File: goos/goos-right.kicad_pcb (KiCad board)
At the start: 2 copper layers, 140.2 x 108.1 mm, 22 parts

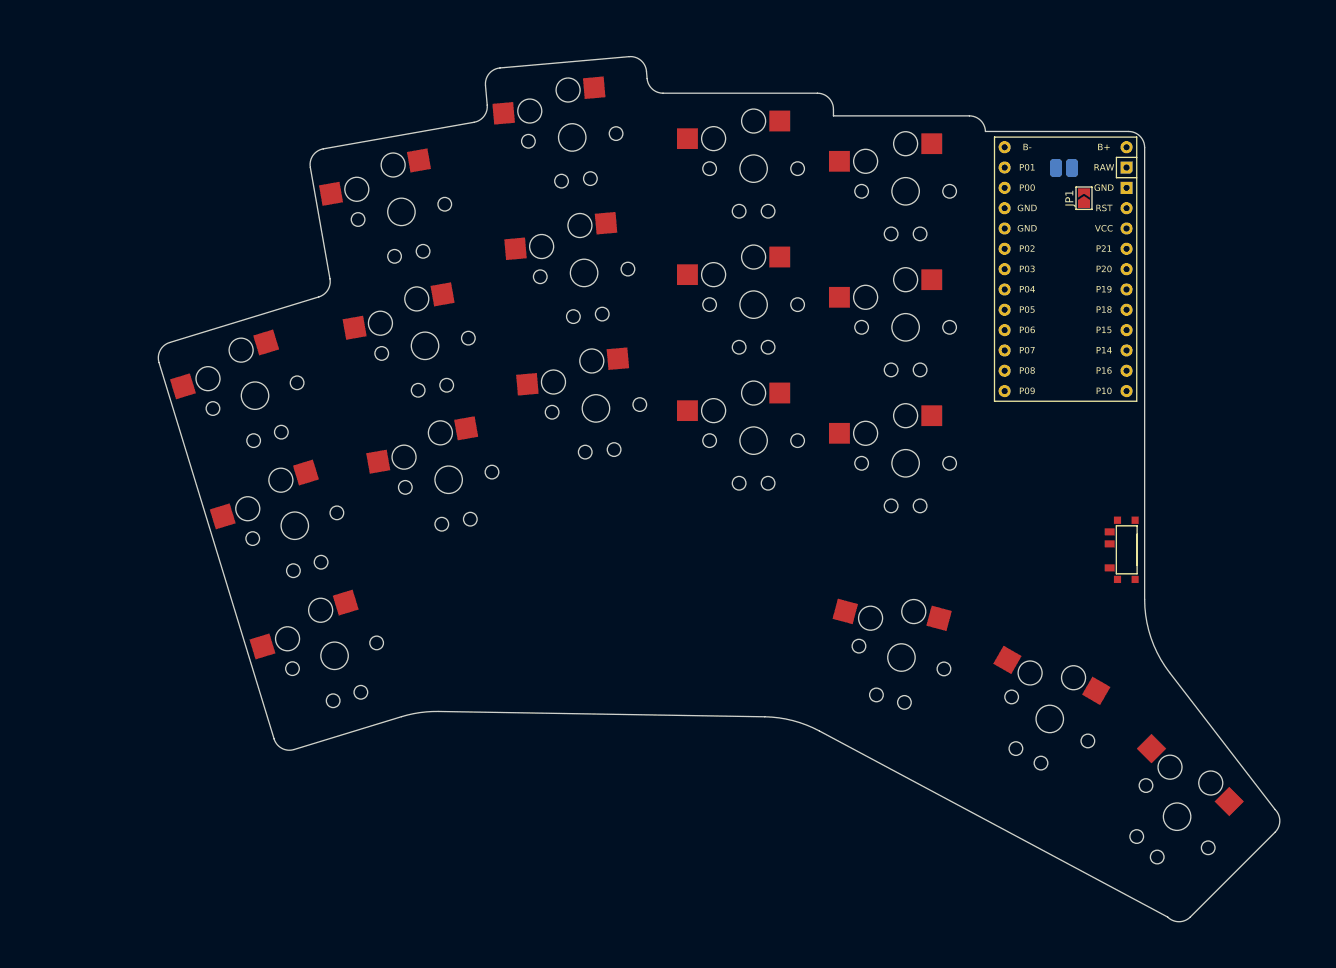
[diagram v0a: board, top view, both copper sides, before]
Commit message: feat: right side routed
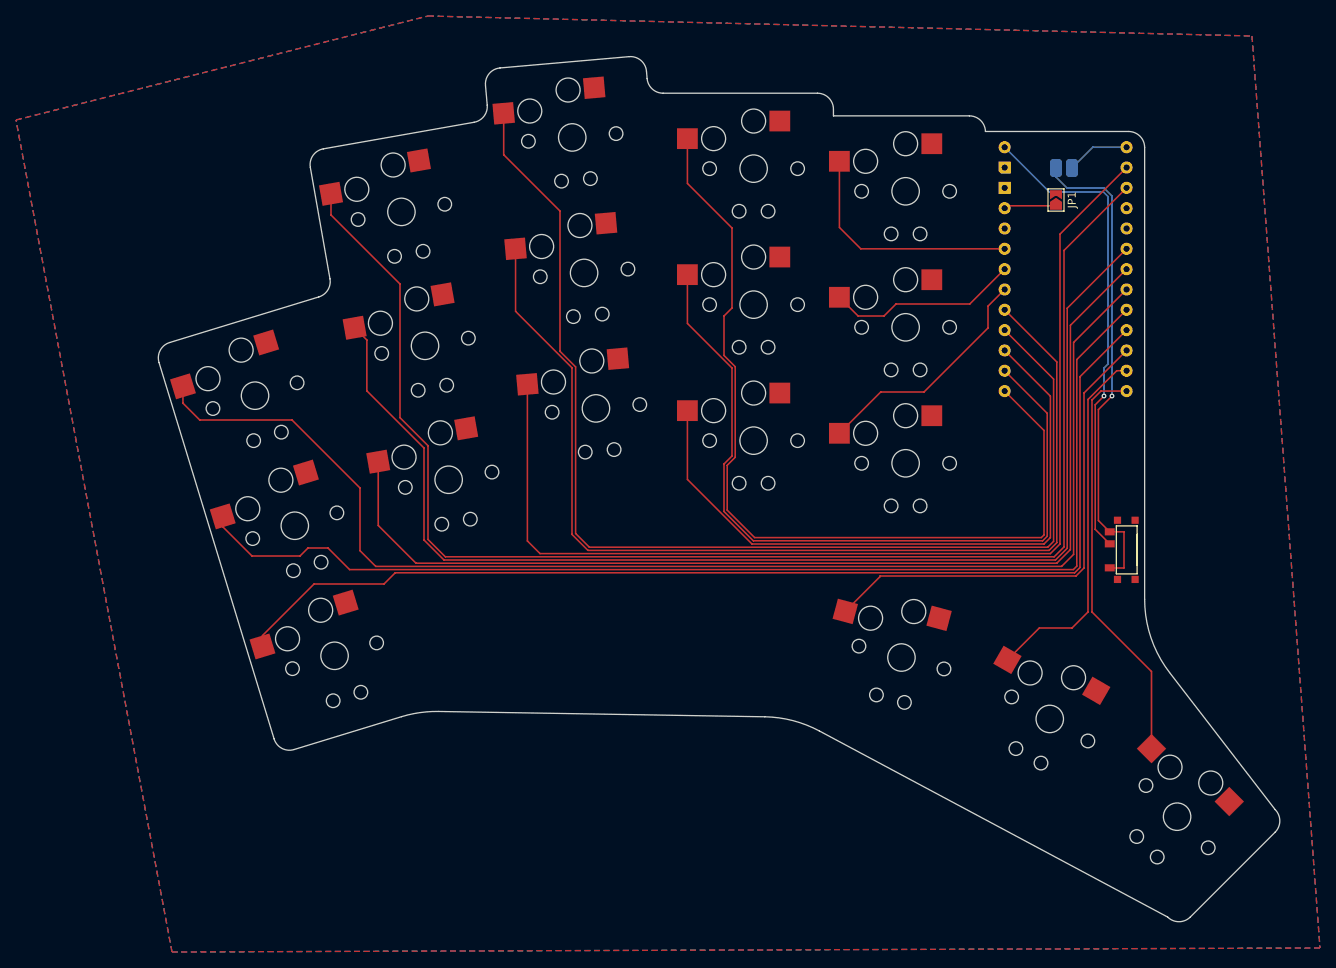
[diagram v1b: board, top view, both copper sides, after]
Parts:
- U1: moved to B.Cu
- moved JP1 3.51 mm to (235.0, 39.5)
- turned J1 to 180 degrees
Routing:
- net D0: track 0.00 -> 177.3 mm
- net D4: track 0.00 -> 163.0 mm
- net D2: track 0.00 -> 152.7 mm
- net D15: track 0.00 -> 145.9 mm
- net D5: track 0.00 -> 145.9 mm
- net D6: track 0.00 -> 139.2 mm
- net D1: track 0.00 -> 137.8 mm
- net D3: track 0.00 -> 135.1 mm
- net D18: track 0.00 -> 132.3 mm
- net D10: track 0.00 -> 111.3 mm
- net D16: track 0.00 -> 97.4 mm
- net D14: track 0.00 -> 83.4 mm
- net D7: track 0.00 -> 61.5 mm
- net Net-(J1-B+): track 0.00 -> 60.5 mm, vias 0 -> 1
- net Net-(U1-B+): track 0.00 -> 60.3 mm, vias 0 -> 1
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- added copper zone on B.Cu, net GND
- added copper zone on F.Cu, net GND
